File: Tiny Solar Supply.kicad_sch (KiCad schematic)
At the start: 16 parts, among them J1 Conn_01x02_Pin, J2 Conn_01x02_Pin, J3 Conn_01x02_Pin, J4 Conn_01x02_Pin, Q1 2N7002, U3 AP3015AKTR-G1

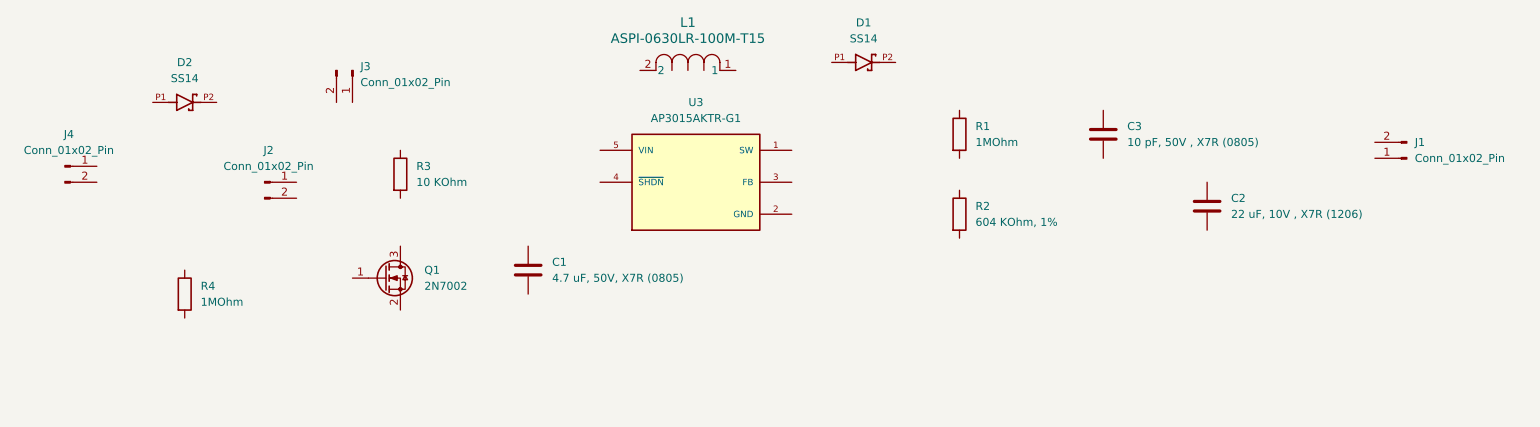
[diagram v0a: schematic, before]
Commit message: Schematic design done
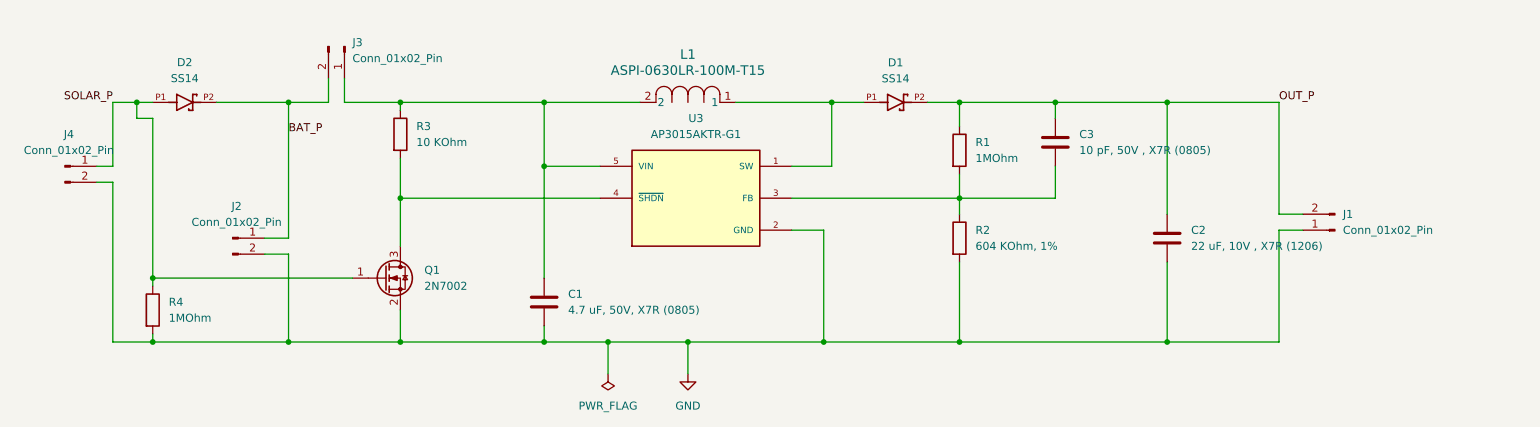
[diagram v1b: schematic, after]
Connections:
- net at R2.1: now also C3.2, R1.2, U3.3 (FB)
- net GND: now reaches R2.2
- net GND: now also C1.2, C2.2, J1.1 (Pin_1), J2.2 (Pin_2), J4.2 (Pin_2), Q1.2 (S), R4.2, U3.2 (GND)
- net at C1.1: now also J3.1 (Pin_1), L1.2, R3.1, U3.5 (VIN)
- net SOLAR_P: now reaches D2.P1
- net SOLAR_P: now also J4.1 (Pin_1), Q1.1 (G), R4.1
- net BAT_P: now reaches D2.P2
- net BAT_P: now also J2.1 (Pin_1), J3.2 (Pin_2)
- net at L1.1: now also D1.P1, U3.1 (SW)
- net OUT_P: now reaches D1.P2
- net OUT_P: now also C2.1, C3.1, J1.2 (Pin_2), R1.1
- net at Q1.3 (D): now also R3.2, U3.4 (~{SHDN})
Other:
- moved on the sheet: C1, C2, C3, D1, J1, J2, J3, L1, R1, R2, R3, R4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
